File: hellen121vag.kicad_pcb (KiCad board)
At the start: 4 copper layers, 164 x 118 mm, 103 parts, among them J21 Conn_01x05_Male, J22 USB_B_Mini, M1 Module-power_12and5V-0.3, M2 Module-knock-0.2, M3 Module-vr-discrete-0.5, M4 Module-vr-max9924-0.1, M5 Module-wbo-0.5, M6 Module:mega-mcu100/0.3, M7 Module-can-0.1, M8 Module-motor-driver-0.1, P1 368255-2, Q1 ISL9V3040D3ST, Q2 ISL9V3040D3ST, Q3 ISL9V3040D3ST, Q4 ISL9V3040D3ST, Q5 ISL9V3040D3ST, Q6 ISL9V3040D3ST, Q7 AO3400A, U10 BTS6143D, U11 VNLD5160TR-E, U3 VNLD5160TR-E, U4 VNLD5160TR-E, U5 VNLD5160TR-E, U6 VNLD5160TR-E, U7 VNLD5160TR-E, U8 MAX31855KASA, U9 VNLD5160TR-E

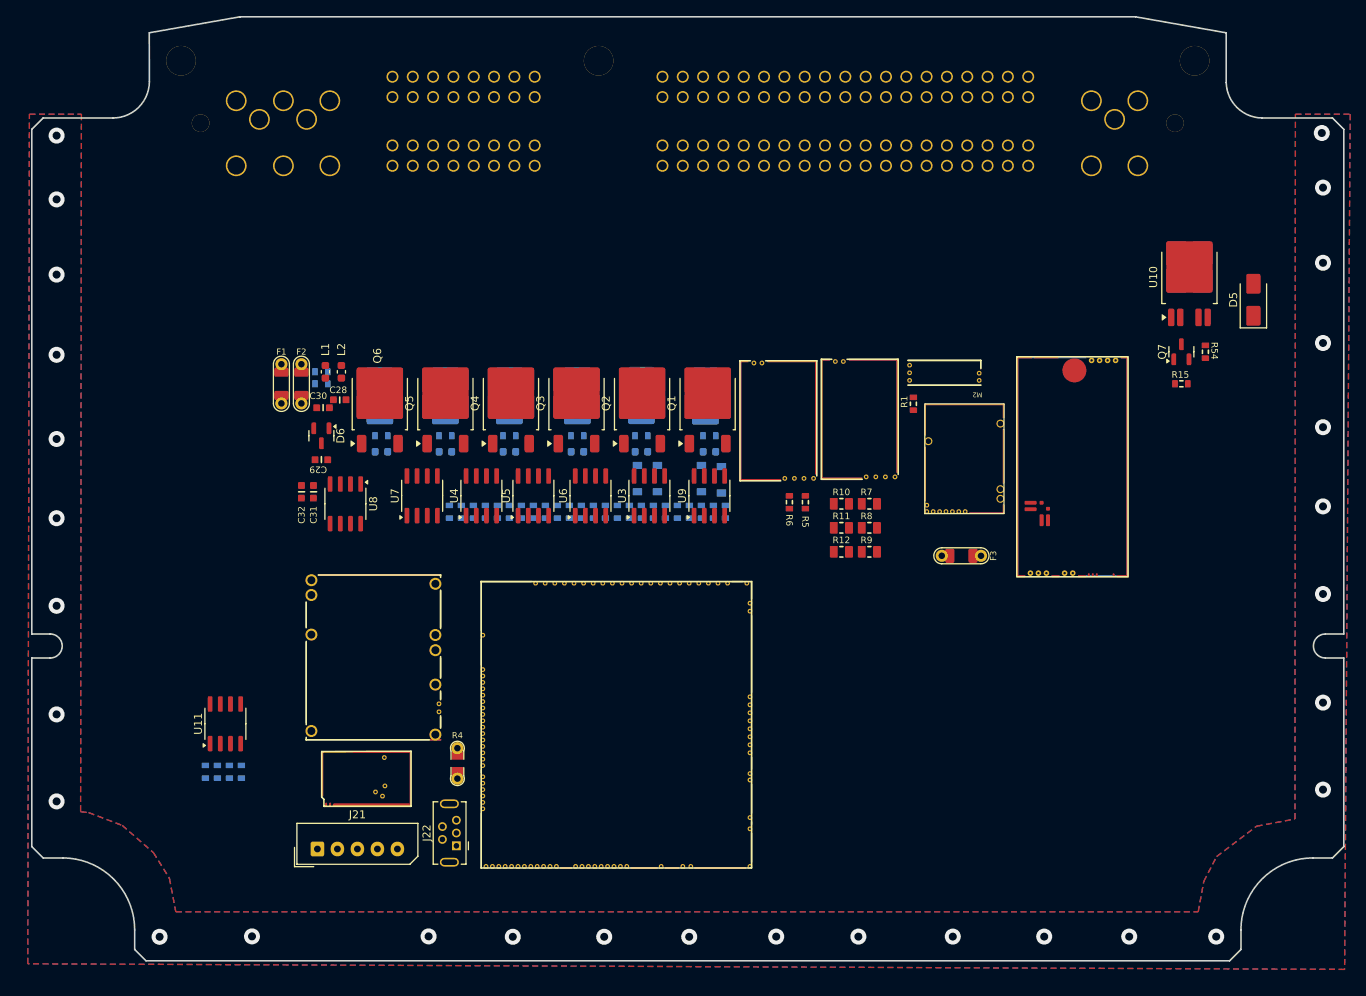
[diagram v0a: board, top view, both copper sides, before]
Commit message: reeeds
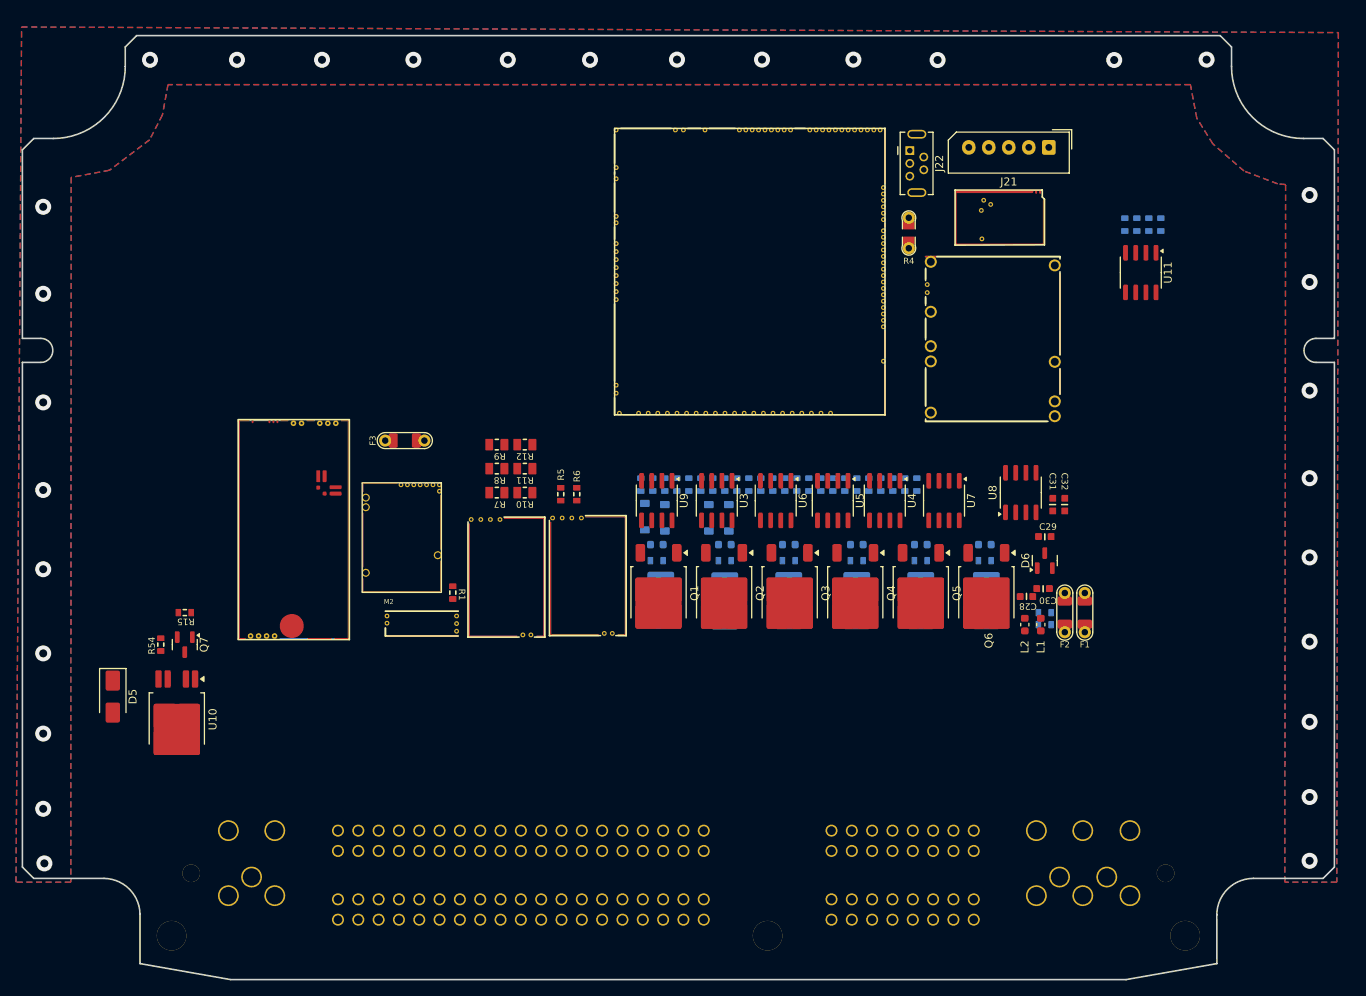
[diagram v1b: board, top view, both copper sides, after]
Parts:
- moved D5 151.0 mm to (55.4, 76.6), turned to -90 degrees
- moved P1 140.5 mm to (58.6, 34.5), turned to 0 degrees
- moved U10 138.1 mm to (63.4, 79.4), turned to -90 degrees
- moved R52 137.6 mm to (186.4, 17.6), turned to -90 degrees
- moved R54 135.6 mm to (61.4, 70.1), turned to 90 degrees
- moved R40 135.0 mm to (184.9, 17.6), turned to -90 degrees
- moved R53 132.5 mm to (183.4, 17.6), turned to -90 degrees
- moved R41 129.9 mm to (181.9, 17.6), turned to -90 degrees
- moved Q7 129.8 mm to (64.4, 70.1), turned to -90 degrees
- moved R15 127.8 mm to (64.4, 66.1), turned to 180 degrees
- moved U11 127.6 mm to (183.9, 23.6), turned to -90 degrees
- moved J21 126.7 mm to (172.4, 7.95), turned to 180 degrees
- moved M7 119.0 mm to (172.0, 13.2), turned to 180 degrees
- moved M5 113.2 mm to (71.0, 41.9), turned to -90 degrees
- moved M1 112.2 mm to (173.9, 21.5), turned to 180 degrees
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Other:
- outline, holes or cut-outs redrawn
